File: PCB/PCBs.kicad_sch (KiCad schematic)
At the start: 4 parts, among them U1 ADS1299IPAGR

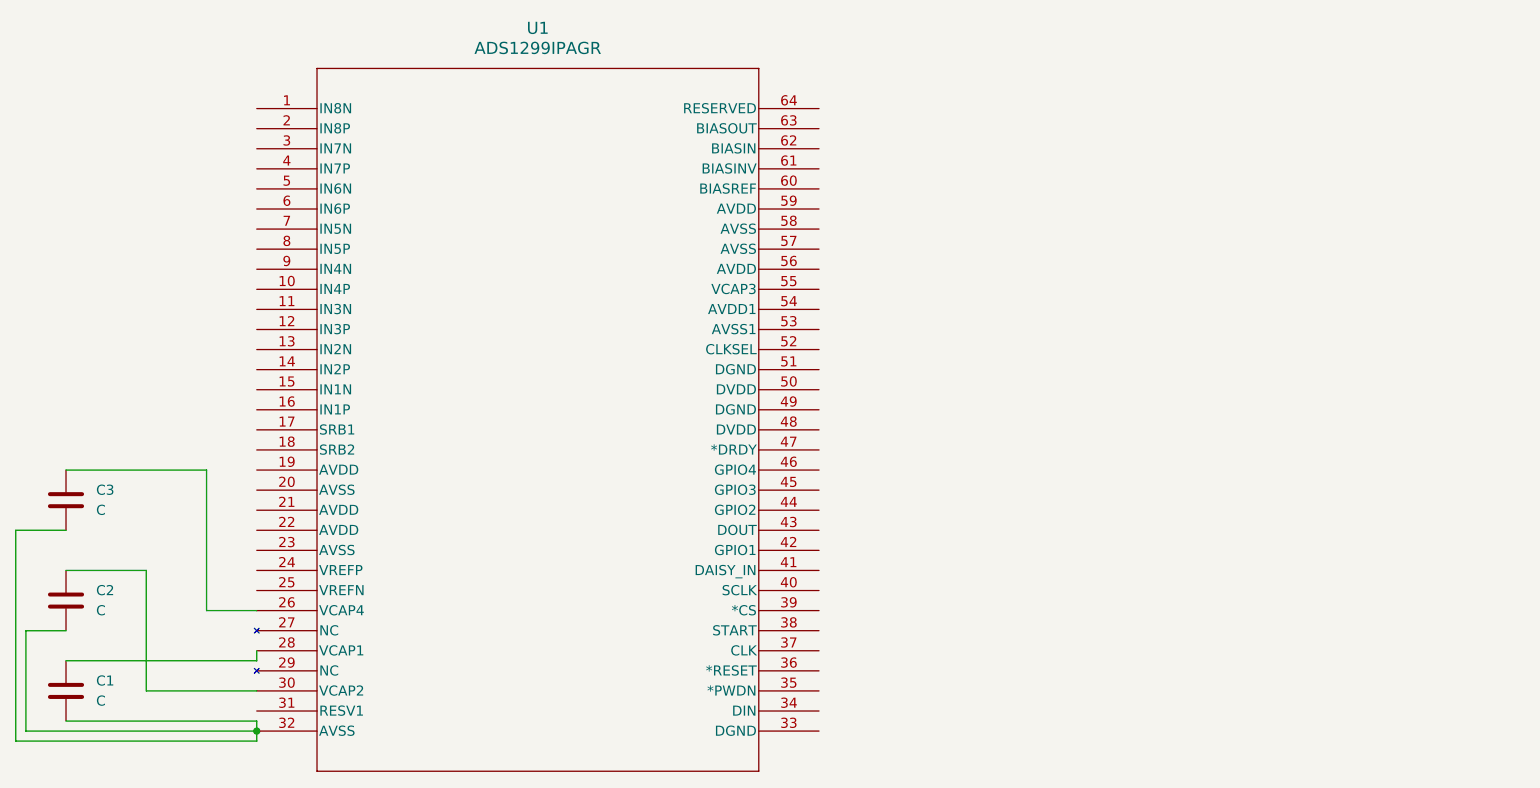
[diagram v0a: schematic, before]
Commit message: moving vcaps
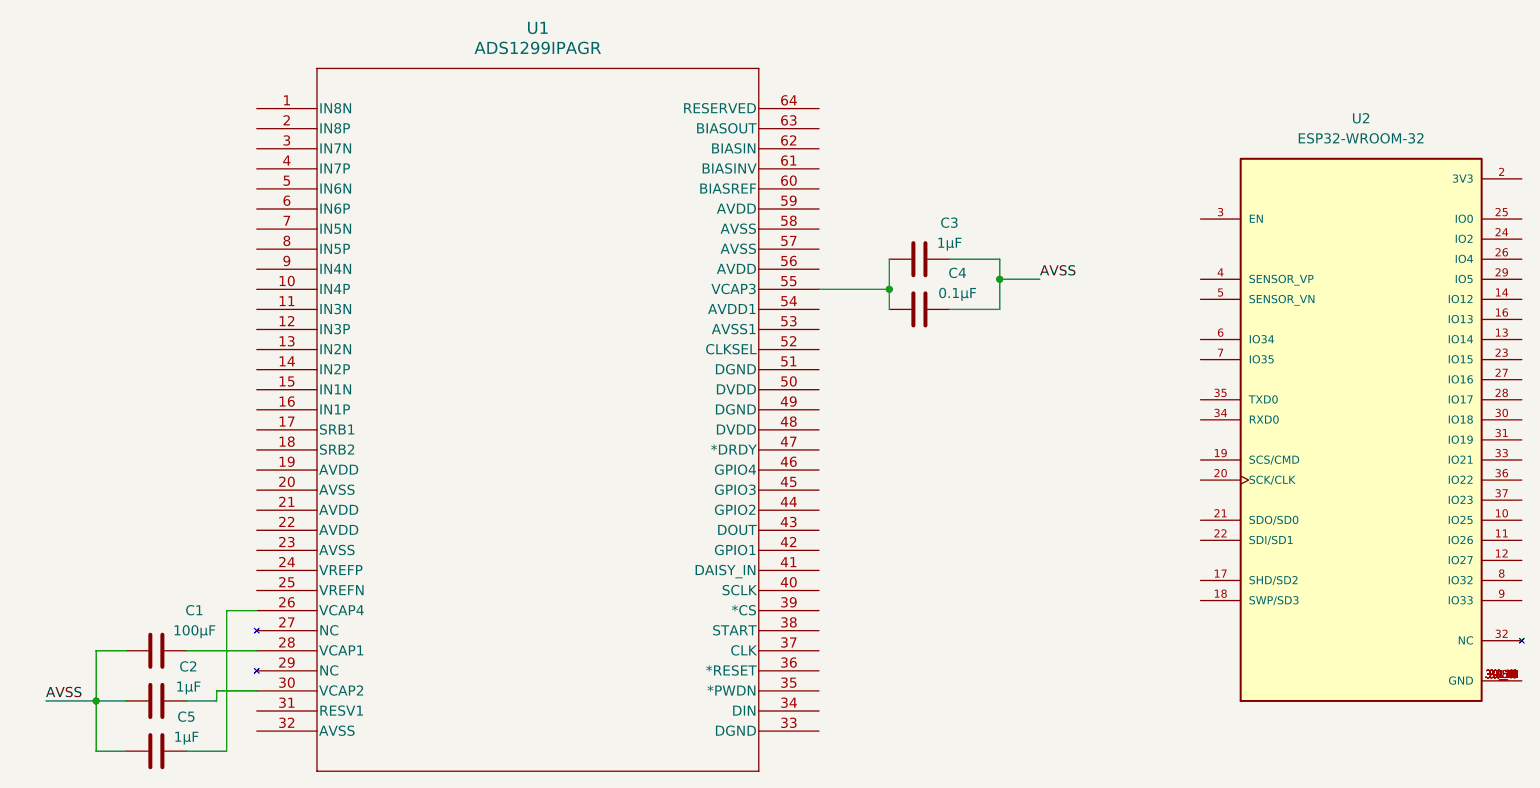
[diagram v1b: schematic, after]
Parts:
- added C4: 0.1µF, symbol Device:C
- added C5: 1µF, symbol Device:C
- added U2: ESP32-WROOM-32, ESP32-WROOM-32:MODULE_ESP32-WROOM-32, symbol custom_lib:ESP32-WROOM-32
- C1: value C -> 100µF
- C2, C3: value C -> 1µF
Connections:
- net at U1.26 (VCAP4): now also C5.1; no longer C3.1
- net AVSS: now reaches C1.2, C2.2
- net AVSS: now also C3.1, C4.1, C5.2; no longer C3.2, U1.32 (AVSS)
- net at U1.55 (VCAP3): now also C3.2, C4.2
- new net: U2.1 (GND), U2.15 (GND), U2.38 (GND), U2.39_1 (GND), U2.39_10 (GND), U2.39_11 (GND), U2.39_12 (GND), U2.39_13 (GND), U2.39_14 (GND), U2.39_15 (GND), U2.39_16 (GND), U2.39_17 (GND), U2.39_18 (GND), U2.39_19 (GND), U2.39_2 (GND), U2.39_20 (GND), U2.39_21 (GND), U2.39_3 (GND), U2.39_4 (GND), U2.39_5 (GND), U2.39_6 (GND), U2.39_7 (GND), U2.39_8 (GND), U2.39_9 (GND)
